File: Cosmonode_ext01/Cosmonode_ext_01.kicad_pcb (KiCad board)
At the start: 2 copper layers, 19.7 x 31.1 mm, 15 parts, among them J1 GS2, J2 GS3, J3 CONN_01X07, J5 CONN_01X07, J7 GS3, J8 GS3, J9 GS3, U1 TSL2561T(6P-3.8X2.6MM), U2 BMP180, U3 SI7020-A20-YM0R

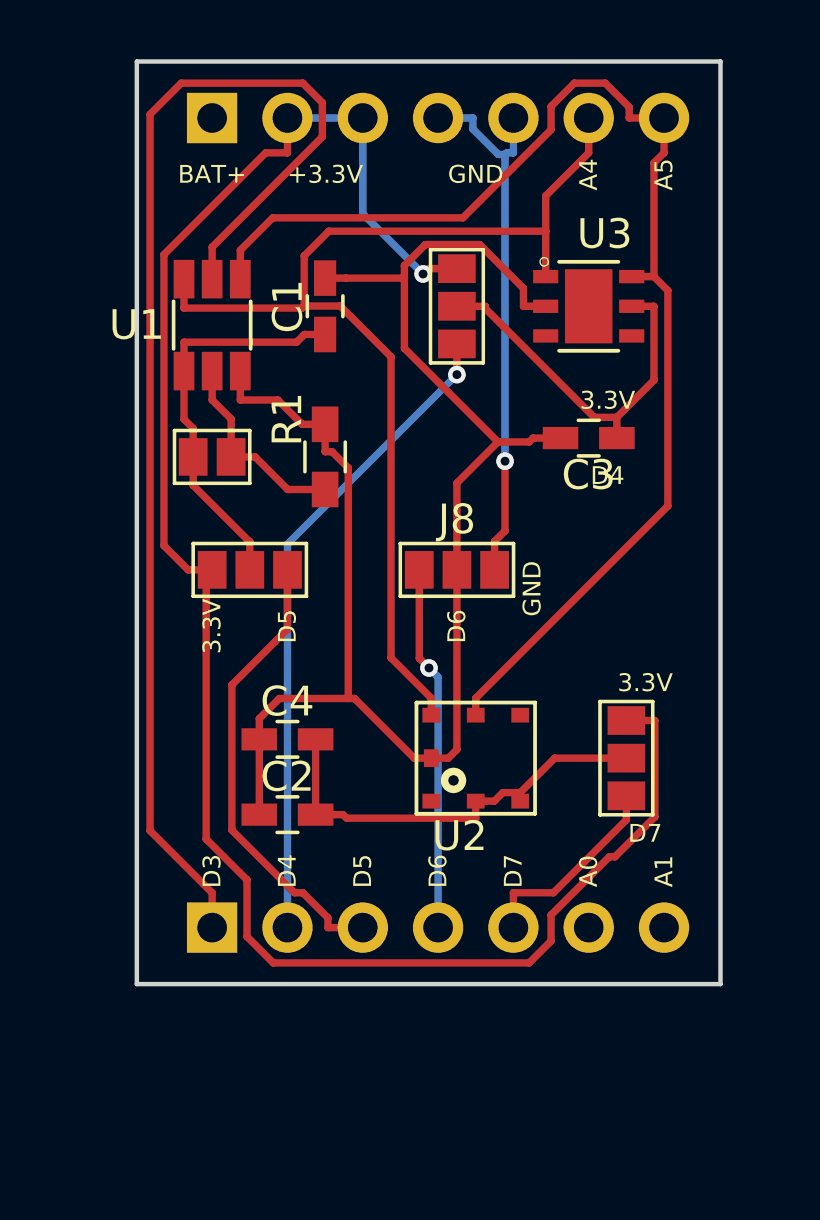
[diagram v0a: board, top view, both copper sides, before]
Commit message: fully update to v0.3
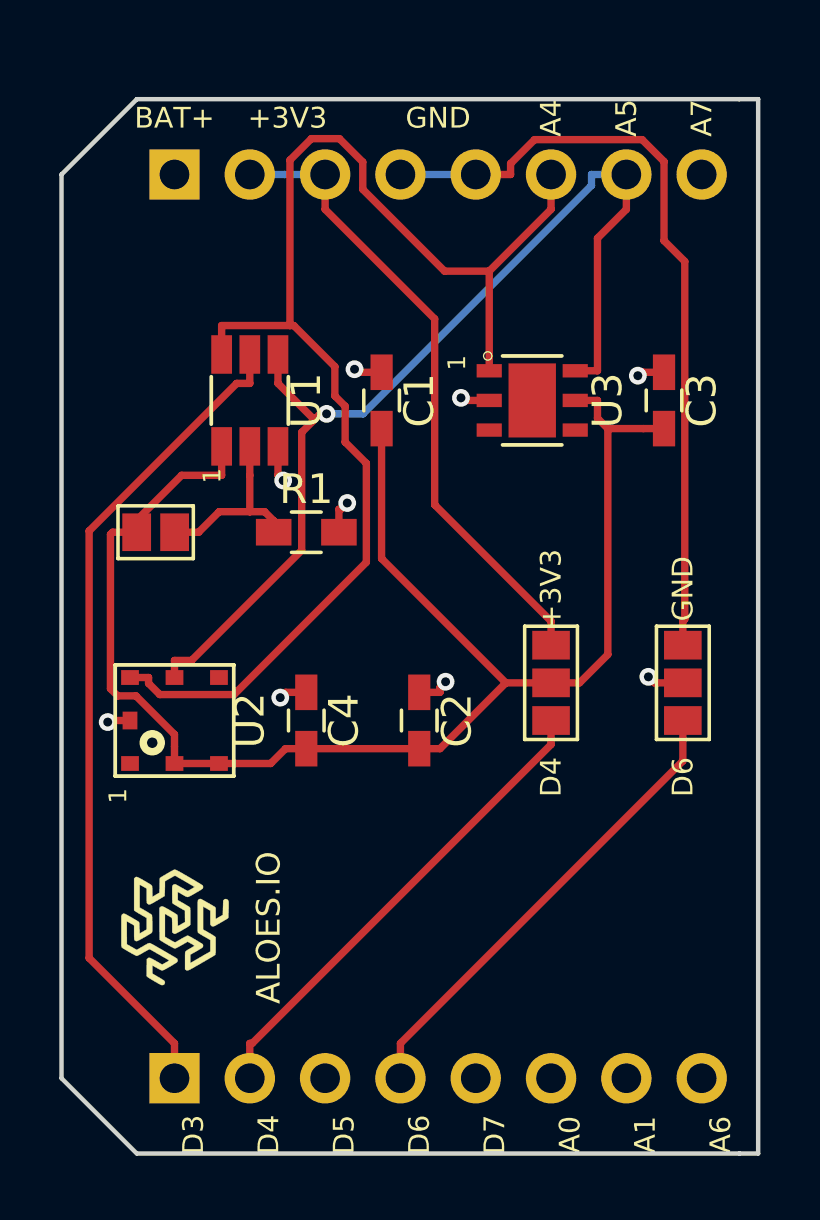
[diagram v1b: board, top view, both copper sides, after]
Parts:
- removed J2, J7: GS3, Connectors:GS3
- added J4: Aloes_Logo, Aloes:Aloes_mini, F.Cu at (167.6, 130.8)
- added J6: OSHW_Logo, Symbols:OSHW-Logo_5.7x6mm_SilkScreen, B.Cu at (168.3, 111.1)
- J3, J5: value CONN_01X07 -> CONN_01X08; footprint Pin_Headers:Pin_Header_Straight_1x07_Pitch2.54mm -> Socket_Strips:Socket_Strip_Straight_1x08_Pitch2.54mm
- U1: footprint TSL2561T_6P-3.8X2.6MM_:TMB6-1.55-3.8X2.6MM -> TSL2561T:TMB6-1.55-3.8X2.6MM
- moved J9 13.1 mm to (180.3, 122.6)
- moved U2 10.2 mm to (167.6, 123.8)
- moved J8 8.52 mm to (184.8, 122.6), turned to 0 degrees
- moved C2 5.46 mm to (175.9, 123.8), turned to 90 degrees
- moved J3 5.24 mm to (167.6, 135.9)
- moved C1 3.70 mm to (174.6, 113.0)
- moved U3 3.70 mm to (179.7, 113.0)
- moved J1 3.17 mm to (167.0, 117.5)
- moved U1 2.84 mm to (170.2, 113.0)
- moved C3 2.84 mm to (184.2, 113.0), turned to 90 degrees
- moved R1 2.62 mm to (172.1, 117.5), turned to 0 degrees
- moved J5 2.29 mm to (167.6, 105.4)
- moved C4 0.90 mm to (172.1, 123.8), turned to 90 degrees
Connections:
- C2 pad 1: Net-(C2-Pad1) -> Net-(C1-Pad1)
- C3 pad 1: Net-(C3-Pad1) -> Net-(C1-Pad1)
- C4 pad 1: Net-(C2-Pad1) -> Net-(C1-Pad1)
- J9 pad 2: Net-(C3-Pad1) -> Net-(C1-Pad1)
- U2 pad 2: Net-(C2-Pad1) -> Net-(C1-Pad1)
- U2 pad 3: Net-(C2-Pad1) -> Net-(C1-Pad1)
- U3 pad 5: Net-(C3-Pad1) -> Net-(C1-Pad1)
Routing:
- net Net-(C1-Pad2): track 54.3 -> 9.35 mm, vias 0 -> 9
- net +3V3: track 62.2 -> 21.6 mm, vias 1 -> 0
- net Net-(C1-Pad1): track 13.5 -> 52.7 mm
- net /D5: track 15.5 -> 0.00 mm
- net Net-(C2-Pad1): track 14.5 -> 0.00 mm
- net /D3: track 42.3 -> 28.1 mm
- net Net-(C3-Pad1): track 12.7 -> 0.00 mm
- net GND: track 18.6 -> 26.5 mm, vias 1 -> 0
- net /A4: track 37.5 -> 45.1 mm
- net /A5: track 42.7 -> 35.6 mm, vias 0 -> 1
- net /D7: track 6.81 -> 0.00 mm
- net /D4: track 22.1 -> 16.3 mm, vias 1 -> 0
- net /D6: track 12.3 -> 16.0 mm, vias 1 -> 0
- added copper zone on B.Cu, net Net-(C1-Pad2)
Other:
- board size 19.7 x 31.1 mm -> 23.5 x 35.6 mm
- board text added: "+3V3"
- board text added: "1"
- board text added: "A6"
- board text added: "A7"
- board text added: "ALOES.IO"
- board text added: "Extension #1 TSL2561 BMP180 Si7021"
- board text removed: "+3.3V"
- board text removed: "3.3V"
